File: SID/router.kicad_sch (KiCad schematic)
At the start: 0 parts

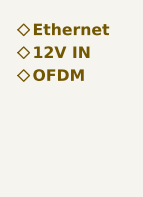
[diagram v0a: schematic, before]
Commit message: Feat(SID): basically complete
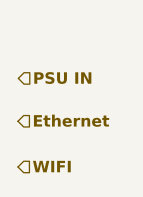
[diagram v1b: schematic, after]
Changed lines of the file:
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@@
 	(generator_version "8.99")
 	(paper "A4")
-	(hierarchical_label "OFDM"
-		(shape bidirectional)
-		(at 109.22 91.44 0)
-		(fields_autoplaced yes)
-		(effects
-			(font
-				(face "JetBrains Mono")
-				(size 1.27 1.27)
-				(thickness 0.254)
-				(bold yes)
-			)
-			(justify left)
-		)
-	)
-	(hierarchical_label "12V IN"
-		(shape bidirectional)
-		(at 109.22 88.9 0)
+	(hierarchical_label "PSU IN"
+		(shape input)
+		(at 109.2592 91.7612 0)
 		(fields_autoplaced yes)
 		(effects
@@
 	)
 	(hierarchical_label "Ethernet"
-		(shape bidirectional)
-		(at 109.22 86.36 0)
+		(shape input)
+		(at 109.22 96.52 0)
 		(fields_autoplaced yes)
 		(effects
+			(font
+				(face "JetBrains Mono")
+				(size 1.27 1.27)
+				(thickness 0.254)
+				(bold yes)
+			)
+			(justify left)
+		)
+	)
+	(hierarchical_label "WIFI"
+		(shape input)
+		(at 109.22 101.6 0)
+		(fields_autoplaced yes)
+		(effects
